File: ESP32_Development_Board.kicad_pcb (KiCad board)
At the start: 2 copper layers, 64.9 x 19.8 mm, 47 parts, among them J1 Conn_01x17_Pin, J2 Conn_01x17_Pin, J3 Conn_01x03_Pin, J4 USB_B_Micro, J5 Conn_01x02_Pin, Q1 NPN, Q2 NPN, Q3 Q_NMOS_GDS, Q4 Q_NMOS_GDS, SW1 SW_Push, SW2 SW_Push, U1 ESP32-WROOM-32E, U2 CP2102N-Axx-xQFN28, U3 AMS1117-3.3

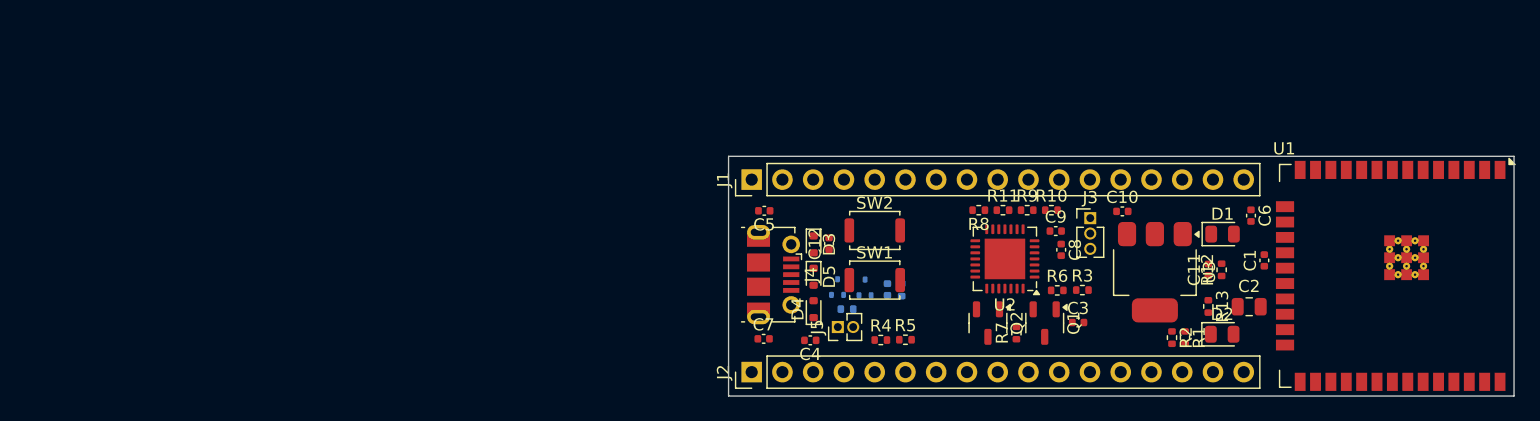
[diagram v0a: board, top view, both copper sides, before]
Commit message: Aug 16, 2025
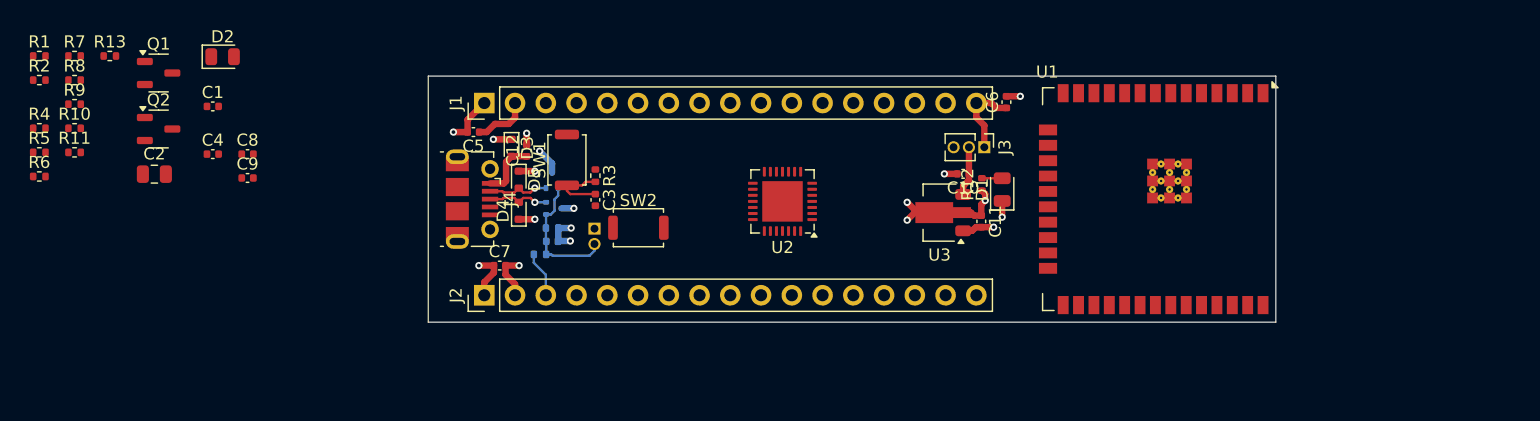
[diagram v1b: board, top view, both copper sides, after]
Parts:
- J5: moved to B.Cu
- U3: footprint Package_TO_SOT_SMD:SOT-223-3_TabPin2 -> Package_TO_SOT_SMD:SOT-89-3
- moved R1 97.4 mm to (76.0, 84.4), turned to 0 degrees
- moved R2 95.9 mm to (76.0, 86.4), turned to 0 degrees
- moved R13 93.1 mm to (81.8, 84.4), turned to 0 degrees
- moved C2 91.1 mm to (85.5, 94.2)
- moved C1 87.8 mm to (90.3, 88.6), turned to 0 degrees
- moved D2 85.7 mm to (91.1, 84.5)
- moved R6 84.6 mm to (76.0, 94.4)
- moved R7 81.1 mm to (78.9, 84.4), turned to 0 degrees
- moved R10 81.0 mm to (78.9, 90.4)
- moved R9 79.2 mm to (78.9, 88.4)
- moved R11 76.8 mm to (78.9, 92.4)
- moved Q1 76.0 mm to (85.8, 85.8), turned to 0 degrees
- moved R8 75.4 mm to (78.9, 86.4), turned to 0 degrees
- moved R5 73.2 mm to (76.0, 92.4)
- moved R4 71.7 mm to (76.0, 90.4)
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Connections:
- D4 pad 2: /USB_DN -> /USB_DP
- D5 pad 2: /USB_DP -> /USB_DN
- J4 pad 2: /USB_DP -> /USB_DN
- J4 pad 3: /USB_DN -> /USB_DP
- Q3 pad 2: /USB_DN -> /USB_DP
- Q4 pad 2: /USB_DP -> /USB_DN
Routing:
- net GND: track 0.00 -> 25.7 mm, vias 0 -> 14
- net +3.3V: track 0.00 -> 22.4 mm, vias 0 -> 4
- net Net-(J5-Pin_2): track 0.00 -> 10.9 mm
- net +5VD: track 0.00 -> 6.58 mm
- net /EN: track 0.00 -> 5.38 mm
- net /USB_DN: track 0.00 -> 5.13 mm, vias 0 -> 1
- net /USB_DP: track 0.00 -> 5.12 mm, vias 0 -> 1
- net +5VA: track 0.00 -> 4.89 mm
- net +5V: track 0.00 -> 4.10 mm
- net /IO23: track 0.00 -> 3.79 mm
- net Net-(D1-A): track 0.00 -> 1.68 mm
- added copper zone on In1.Cu, net +3.3V
- added copper zone on In2.Cu, net GND
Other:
- board size 64.9 x 19.8 mm -> 70 x 20.3 mm
- copper layers 2 -> 4
